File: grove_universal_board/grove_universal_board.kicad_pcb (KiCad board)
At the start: 2 copper layers, 30.5 x 22.9 mm, 24 parts, among them M2 Hole_M2_2.0

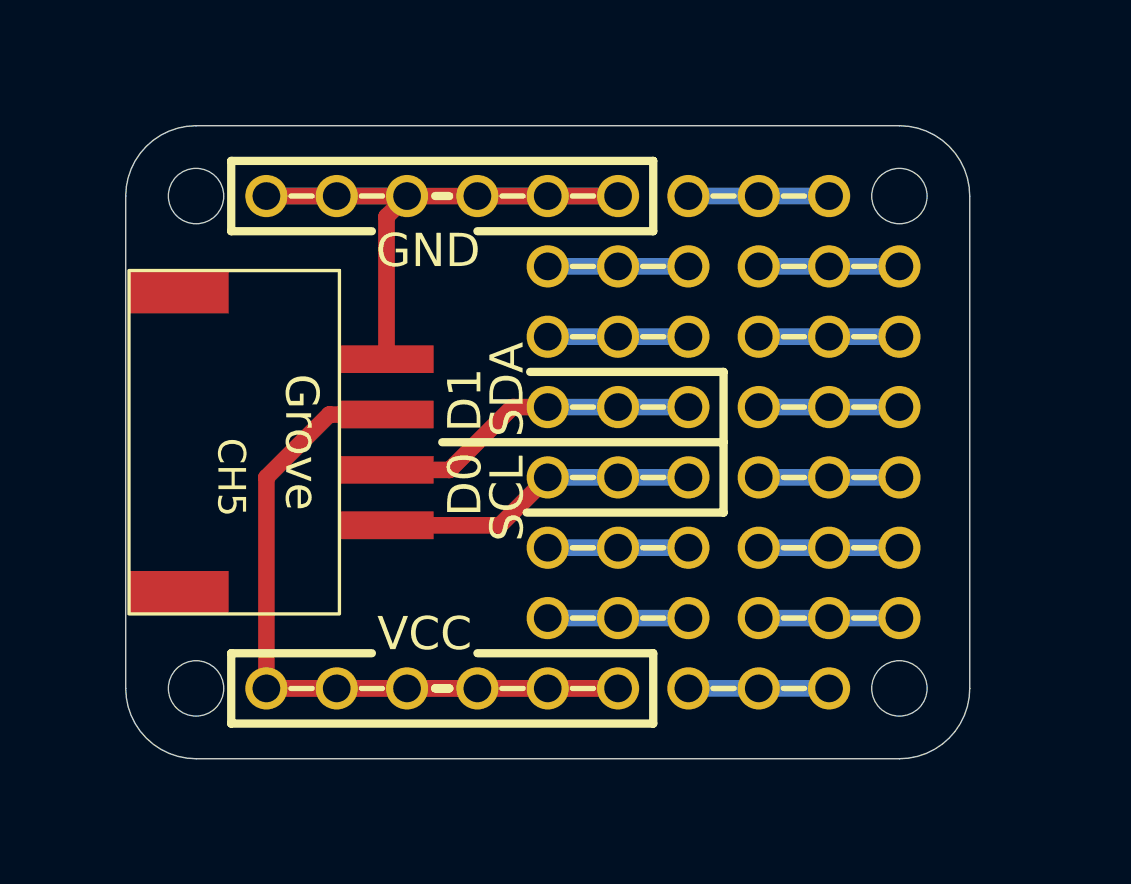
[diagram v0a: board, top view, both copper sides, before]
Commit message: grove_universal_board/v1.1.0
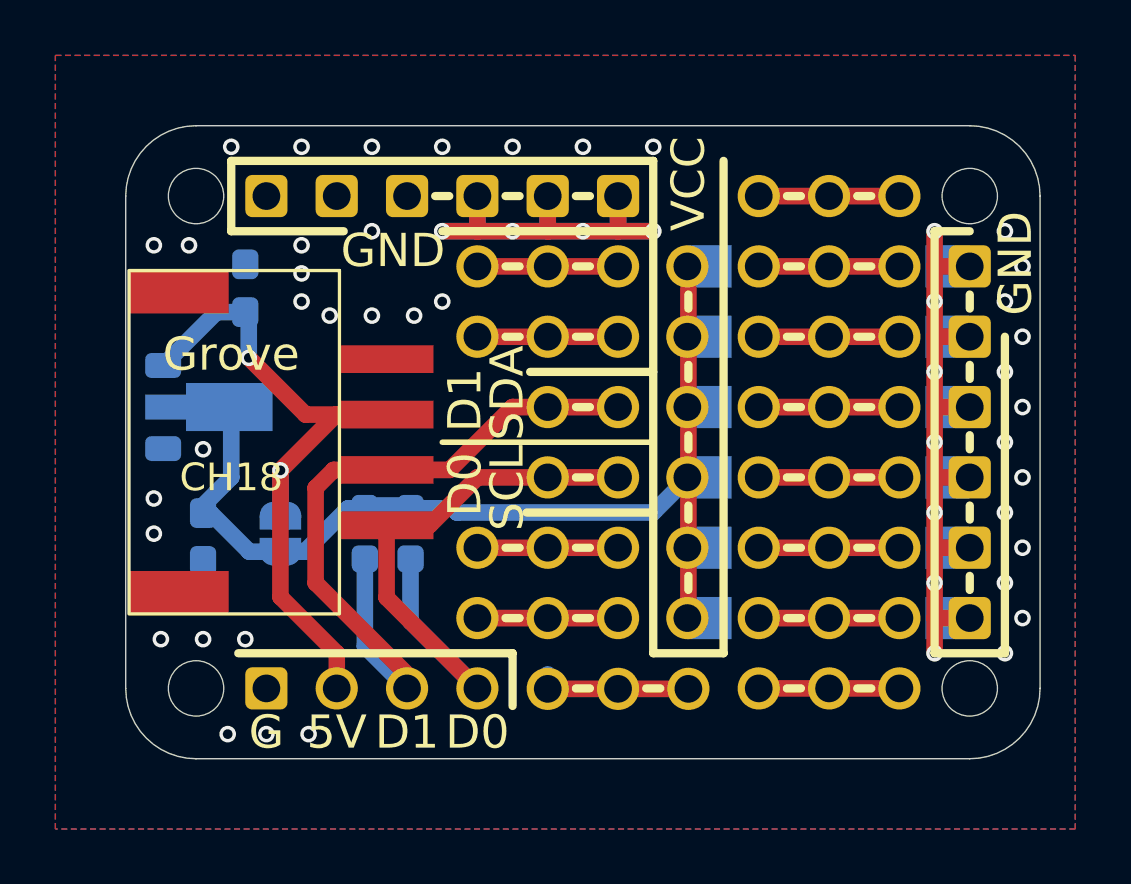
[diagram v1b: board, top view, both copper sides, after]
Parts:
- removed REF** (x12): PinOut_Universal-Board_bridge3, 74th:PinOut_Universal-Board_bridge3
- added C1: 10u, 74th:Capacitor_0603_1608, B.Cu at (91.7, 73.2)
- added C2: 10u, 74th:Capacitor_0603_1608, B.Cu at (93.2, 64.4)
- added CH1: Pin_1, 74th:PinOut_Pin_3, F.Cu at (111.8, 78.7)
- added CH13: Pin_1, 74th:PinOut_Pin_3, F.Cu at (101.6, 76.2)
- added CH14: Pin_1, 74th:PinOut_Pin_3, F.Cu at (101.6, 73.7)
- added CH15: Pin_1, 74th:PinOut_Pin_3, F.Cu at (101.6, 66.0)
- added CH16: Pin_1, 74th:PinOut_Pin_3, F.Cu at (101.6, 63.5)
- added CH17: Pin_1, 74th:PinOut_Pin_3_Square, F.Cu at (101.6, 61.0)
- added CH2: Pin_1, 74th:PinOut_Pin_3, F.Cu at (111.8, 76.2)
- added CH3: Pin_1, 74th:PinOut_Pin_3, F.Cu at (111.8, 73.7)
- added CH4: Pin_1, 74th:PinOut_Pin_3, F.Cu at (111.8, 71.1)
- added CH5: Pin_1, 74th:PinOut_Pin_3, F.Cu at (111.8, 68.6)
- added CH6: Pin_1, 74th:PinOut_Pin_3, F.Cu at (111.8, 66.0)
- added CH7: Pin_1, 74th:PinOut_Pin_3, F.Cu at (111.8, 63.5)
- added CH8: Pin_1, 74th:PinOut_Pin_3, F.Cu at (111.8, 61.0)
- added CH9: Pin_1, 74th:PinOut_Pin_3, F.Cu at (104.1, 78.8)
- added JP1: Jumper_2_Open, 74th:SolderJumper-2, B.Cu at (94.5, 73.2)
- added R1: 1k, 74th:Register_0603_1608, B.Cu at (97.5, 73.2)
- added R2: 1k, 74th:Register_0603_1608, B.Cu at (99.2, 73.2)
- added U1: AMS1117, Package_TO_SOT_SMD:SOT-89-3, B.Cu at (92.2, 68.6)
- CH10: renamed from CH2; footprint 74th:PinOut_Universal-Board_bridge3 -> 74th:PinOut_Pin_2
- CH11: renamed from CH3; footprint 74th:PinOut_Universal-Board_bridge3 -> 74th:PinOut_Pin_2
- CH12: renamed from CH1; footprint 74th:PinOut_Universal-Board_bridge3 -> 74th:PinOut_Pin_4_GND
- CH19: renamed from CH4; footprint 74th:PinOut_Universal-Board_bridge3 -> 74th:PinOut_Pin_3_Square
- CH20: renamed from CH6; footprint 74th:PinOut_Universal-Board_bridge3 -> 74th:PinOut_Universal-Board_bridge6_with-Jumper; moved to B.Cu
- CH21: renamed from CH7; footprint 74th:PinOut_Universal-Board_bridge3 -> 74th:PinOut_Universal-Board_bridge6_with-Jumper_Square; moved to B.Cu
- moved CH21 15.5 mm to (119.4, 63.5), turned to -90 degrees
- moved MISC-ICON 9.26 mm to (96.7, 65.3)
- moved CH20 5.65 mm to (109.2, 76.2), turned to 90 degrees
- moved CH12 5.08 mm to (101.6, 78.7), turned to 180 degrees
- moved CH10 2.54 mm to (104.1, 71.1)
- moved CH11 2.54 mm to (104.1, 68.6)
- moved CH19 2.54 mm to (94.0, 61.0)
- moved M1 2.54 mm to (119.4, 78.7)
- moved M2 2.54 mm to (119.4, 61.0)
- renumbered CH5 to CH18, M2 to M1, M2 to M3, M2 to M4
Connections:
- CH10 pad 1: Net-(CH5-SCL) -> /D0/SCL
- CH11 pad 1: Net-(CH5-SDA) -> /D1/SDA
- CH12 pad 1: Net-(CH5-VCC) -> /D0/SCL
- CH18 pad 1: Net-(CH5-SCL) -> /D0/SCL
- CH18 pad 2: Net-(CH5-SDA) -> /D1/SDA
- CH18 pad 3: Net-(CH5-VCC) -> +5V
- CH18 pad 4: Net-(CH5-GND) -> GND
- CH19 pad 1: Net-(CH5-GND) -> GND
- CH20 pad 1: Net-(CH5-VCC) -> VCC
- CH21 pad 1: Net-(CH5-GND) -> GND
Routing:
- net (no net): track 61.0 -> 0.00 mm
- net GND: track 0.00 -> 45.7 mm, vias 0 -> 50
- net Net-(CH5-VCC): track 38.3 -> 0.00 mm
- net VCC: track 0.00 -> 37.2 mm
- net Net-(CH5-GND): track 29.1 -> 0.00 mm
- net /D1/SDA: track 0.00 -> 26.4 mm
- net +5V: track 0.00 -> 26.3 mm, vias 0 -> 2
- net /D0/SCL: track 0.00 -> 22.4 mm
- net Net-(CH5-SDA): track 12.2 -> 0.00 mm
- net Net-(CH5-SCL): track 12.0 -> 0.00 mm
- net Net-(CH13-Pad1): track 0.00 -> 5.59 mm
- net unconnected-(CH9-Pad1): track 0.00 -> 5.08 mm
- net Net-(CH8-Pad1): track 0.00 -> 5.08 mm
- net Net-(CH11-Pad1): track 0.00 -> 5.08 mm
- net Net-(CH10-Pad1): track 0.00 -> 5.08 mm
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- added copper zone on B.Cu, net GND
- added copper zone on F.Cu, net GND
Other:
- board size 30.5 x 22.9 mm -> 33 x 22.9 mm
- board text added: "5V"
- board text added: "74th-G050-v1.1.0"
- board text added: "G"
- board text added: "Grove UBoard"
- board text removed: "74th-G050-v1.0.0"
- board text removed: "Grove Universal Board"
